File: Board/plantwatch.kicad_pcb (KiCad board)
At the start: 2 copper layers, 159.9 x 101.1 mm, 41 parts, among them IC1 HS1101, J1 Motor Connector, J2 Sensor Connector, J5 nRF24L01P Connector, Q1 BSP129, SW1 SW_Push, SW2 SW_Push, U1 MKL25Z128VLK4, U2 TMP36, U4 NCP1117-3.3_SOT223, Y1 Crystal_GND24

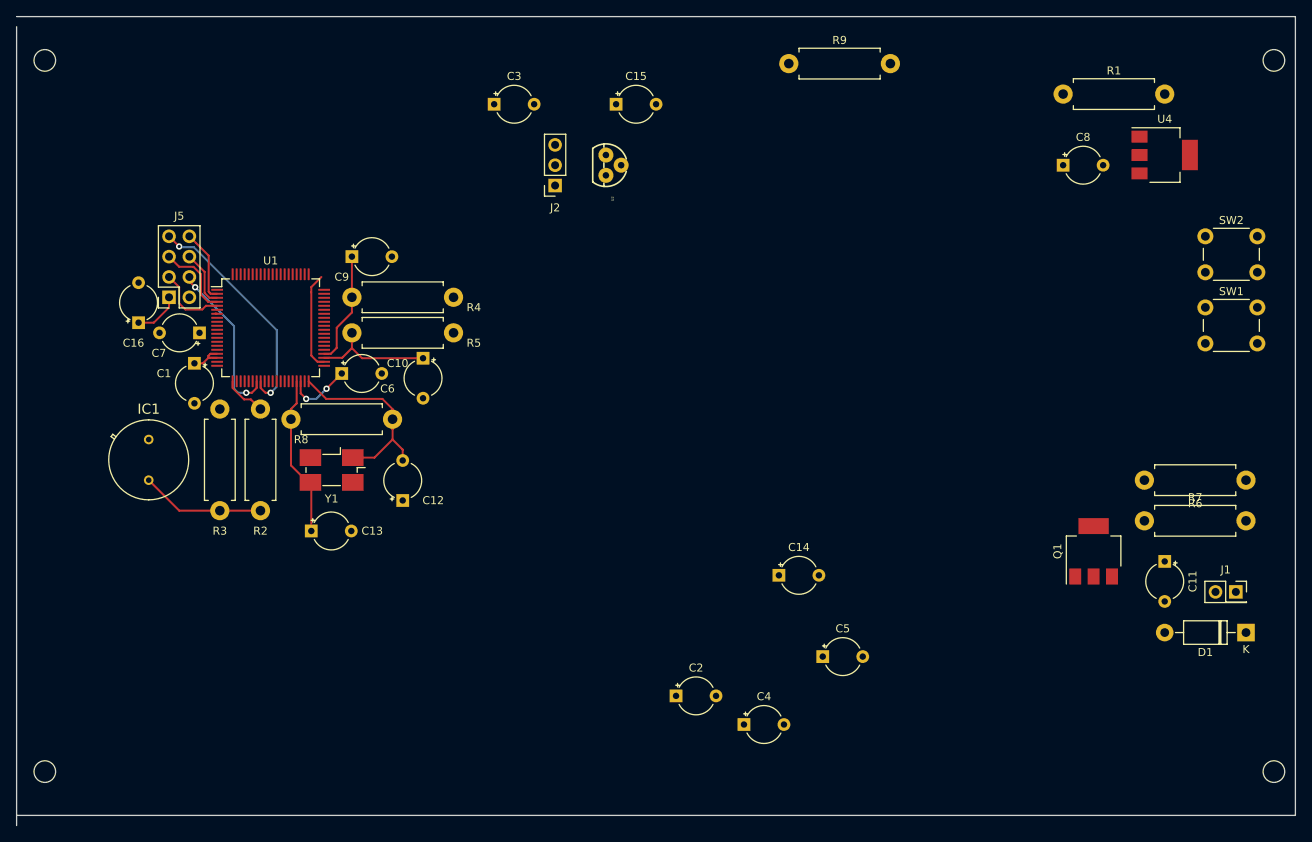
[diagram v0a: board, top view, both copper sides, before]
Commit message: PCB almost done
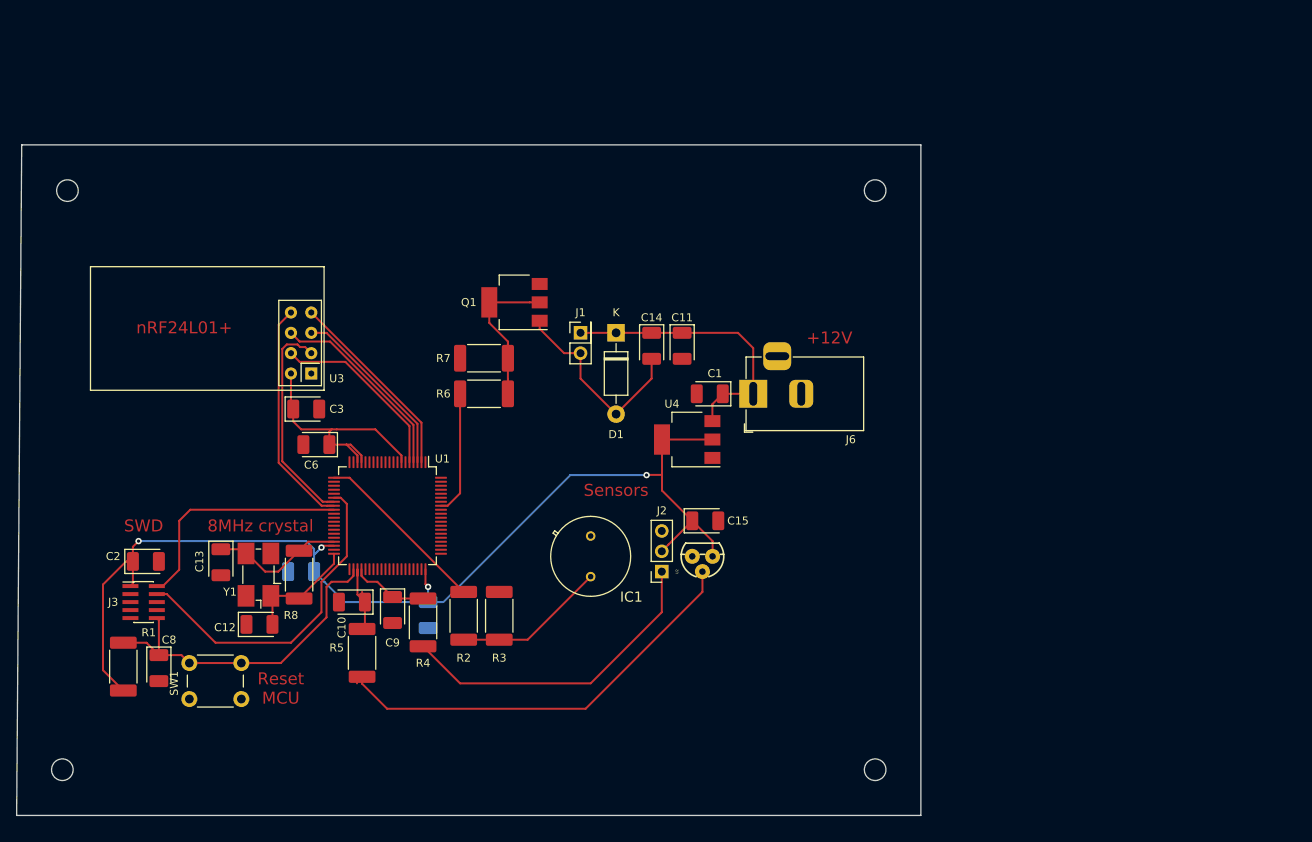
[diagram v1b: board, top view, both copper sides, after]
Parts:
- removed C16: C_Small, Capacitor_THT:CP_Radial_Tantal_D4.5mm_P5.00mm
- removed C7: 0.2uF, Capacitor_THT:CP_Radial_Tantal_D4.5mm_P5.00mm
- removed J5: nRF24L01P Connector, Connector_PinSocket_2.54mm:PinSocket_2x04_P2.54mm_Vertical
- removed R9: 10K, Resistor_THT:R_Axial_DIN0411_L9.9mm_D3.6mm_P12.70mm_Horizontal
- removed SW2: SW_Push, Button_Switch_THT:SW_PUSH_6mm
- added J3: SWD, Connector_PinHeader_1.00mm:PinHeader_2x05_P1.00mm_Vertical_SMD, F.Cu at (71.0, 118.3)
- added J6: Power Input, Connector_BarrelJack:BarrelJack_Horizontal, F.Cu at (147.2, 92.2)
- added U3: nRF24L01+, RF_Module:nRF24L01_Breakout, F.Cu at (91.9, 89.7)
- C1: value 0.2uF -> 0.1uF; footprint Capacitor_THT:CP_Radial_Tantal_D4.5mm_P5.00mm -> Capacitor_Tantalum_SMD:CP_EIA-3528-15_AVX-H_Pad1.50x2.35mm_HandSolder
- C10, C11, C12, C13, C8, C9: footprint Capacitor_THT:CP_Radial_Tantal_D4.5mm_P5.00mm -> Capacitor_Tantalum_SMD:CP_EIA-3528-15_AVX-H_Pad1.50x2.35mm_HandSolder
- C14: value 1uF -> 0.1uF; footprint Capacitor_THT:CP_Radial_Tantal_D4.5mm_P5.00mm -> Capacitor_Tantalum_SMD:CP_EIA-3528-15_AVX-H_Pad1.50x2.35mm_HandSolder
- C15, C2, C3, C6: value C_Small -> 0.1uF; footprint Capacitor_THT:CP_Radial_Tantal_D4.5mm_P5.00mm -> Capacitor_Tantalum_SMD:CP_EIA-3528-15_AVX-H_Pad1.50x2.35mm_HandSolder
- C4, C5: value C_Small -> 0.1uF; footprint Capacitor_THT:CP_Radial_Tantal_D4.5mm_P5.00mm -> Capacitor_Tantalum_SMD:CP_EIA-3528-15_AVX-H_Pad1.50x2.35mm_HandSolder; moved to B.Cu
- J1: value Motor Connector -> Motor
- J2: value Sensor Connector -> SEN0193
- R1, R2, R3, R4, R5, R6, R7, R8: footprint Resistor_THT:R_Axial_DIN0411_L9.9mm_D3.6mm_P12.70mm_Horizontal -> Resistor_SMD:R_2512_6332Metric_Pad1.52x3.35mm_HandSolder
- SW1: value SW_Push -> Reset
- U4: value NCP1117-3.3_SOT223 -> +12V Regulator
- Y1: value Crystal_GND24 -> 8 MHz
- moved R1 137.6 mm to (68.4, 126.3), turned to 90 degrees
- moved SW1 134.6 mm to (76.7, 125.9)
- moved C8 129.3 mm to (72.9, 126.5), turned to 270 degrees
- moved R6 95.9 mm to (113.5, 92.2), turned to 0 degrees
- moved J1 88.1 mm to (125.6, 84.6), turned to 90 degrees
- moved D1 87.2 mm to (130.0, 84.6), turned to 270 degrees
- moved R7 85.0 mm to (113.5, 87.8), turned to 180 degrees
- moved Q1 78.8 mm to (117.3, 80.8), turned to 180 degrees
- moved U4 69.5 mm to (138.9, 97.9), turned to 180 degrees
- moved C2 68.4 mm to (71.2, 113.2)
- moved C11 66.1 mm to (138.3, 86.2)
- moved C1 64.5 mm to (141.7, 92.2), turned to 180 degrees
- moved C4 58.6 mm to (90.6, 114.5), turned to 180 degrees
- moved IC1 56.5 mm to (126.8, 110.0)
- moved C15 53.3 mm to (141.2, 108.1)
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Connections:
- C1 pad 1: +3V3 -> +12V
- C14 pad 1: Net-(C14-Pad1) -> +12V
- C14 pad 2: GND -> Net-(C14-Pad2)
- D1 pad 2: GND -> Net-(C14-Pad2)
- J1 pad 2: GND -> Net-(C14-Pad2)
- Q1 pad 1: GND -> Net-(C14-Pad2)
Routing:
- net +3V3: track 18.9 -> 171.1 mm, vias 2 -> 4
- net Net-(R5-Pad2): track 0.00 -> 54.1 mm
- net Net-(J3-Pad4): track 0.00 -> 41.5 mm
- net Net-(J2-Pad1): track 0.00 -> 40.5 mm
- net +12V: track 0.00 -> 35.9 mm
- net Net-(C8-Pad1): track 12.3 -> 42.8 mm
- net Net-(J3-Pad2): track 0.00 -> 29.7 mm
- net Net-(C14-Pad2): track 0.00 -> 25.6 mm
- net Net-(Q1-Pad2): track 0.00 -> 21.4 mm
- net HS1101: track 5.41 -> 22.1 mm
- net NRF24L01P_SCK: track 7.15 -> 22.8 mm
- net MOTOR: track 0.00 -> 15.5 mm
- net NRF24L01P_MISO: track 9.11 -> 24.4 mm
- net NRF24L01P_MOSI: track 9.84 -> 24.7 mm
- net NRF24L01P_CSN: track 9.08 -> 23.1 mm
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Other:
- board size 159.9 x 101.1 mm -> 113 x 83.8 mm
- board text added: "+12V"
- board text added: "8MHz crystal"
- board text added: "Reset MCU"
- board text added: "SWD"
- board text added: "Sensors"
- board text added: "nRF24L01+"
